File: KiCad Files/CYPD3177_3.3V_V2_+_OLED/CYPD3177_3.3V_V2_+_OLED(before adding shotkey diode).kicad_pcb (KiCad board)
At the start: 4 copper layers, 64 x 17 mm, 94 parts, among them IC1 TPS16630RGER, IC2 TPS22992SRXNR, J1 USB_C_USB2.0_16P, J2 Conn_01x02_Pin, J3 Conn_02x05_Odd_Even, J4 Conn_02x05_Odd_Even, J5 0.91 OLED, J6 QWIIC, J7 Conn_01x05, J8 I2C_Header, Q1 DMC2990UDJ-7, SW1 GT-TC0060-H050-L1, SW2 B3U-1000P, U1 TCA9406DC, U2 INA238, U3 XC6220B331PR-G, U4 TPS62933DRLR, U5 AON7534, U6 AP33772S, U7 AON7534, U8 TPS2117DRL, U9 ATtiny3217-M

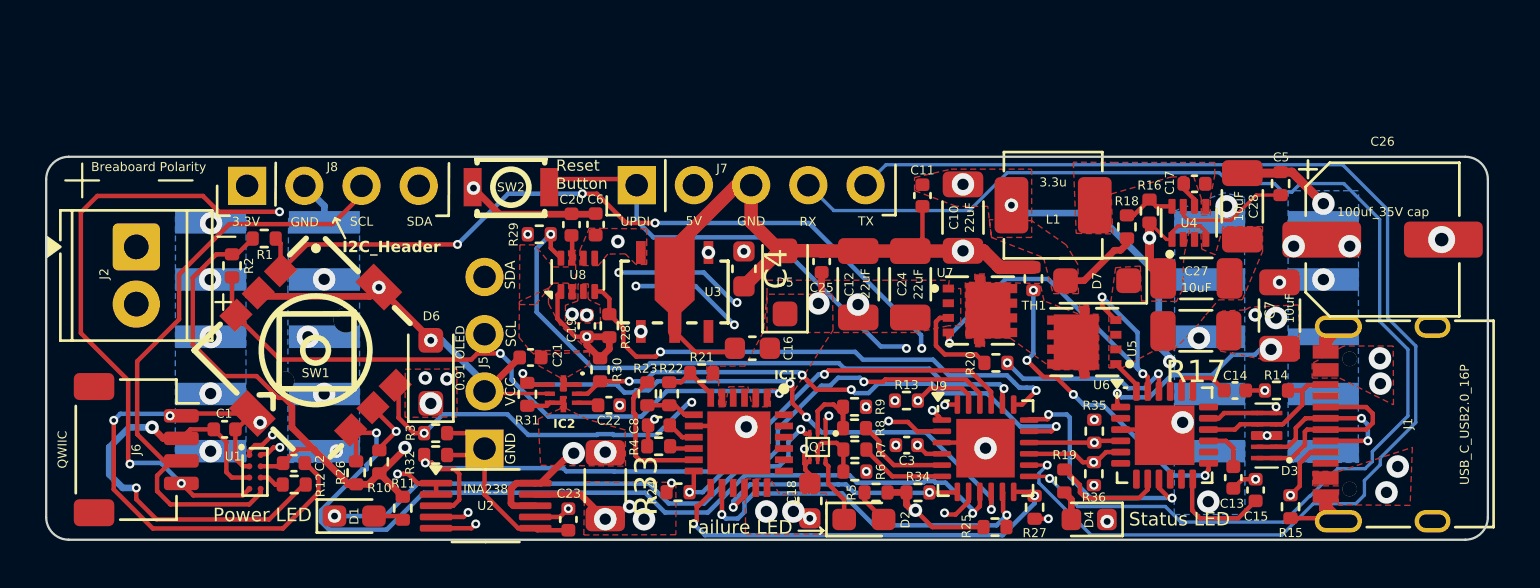
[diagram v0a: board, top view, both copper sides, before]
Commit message: changes
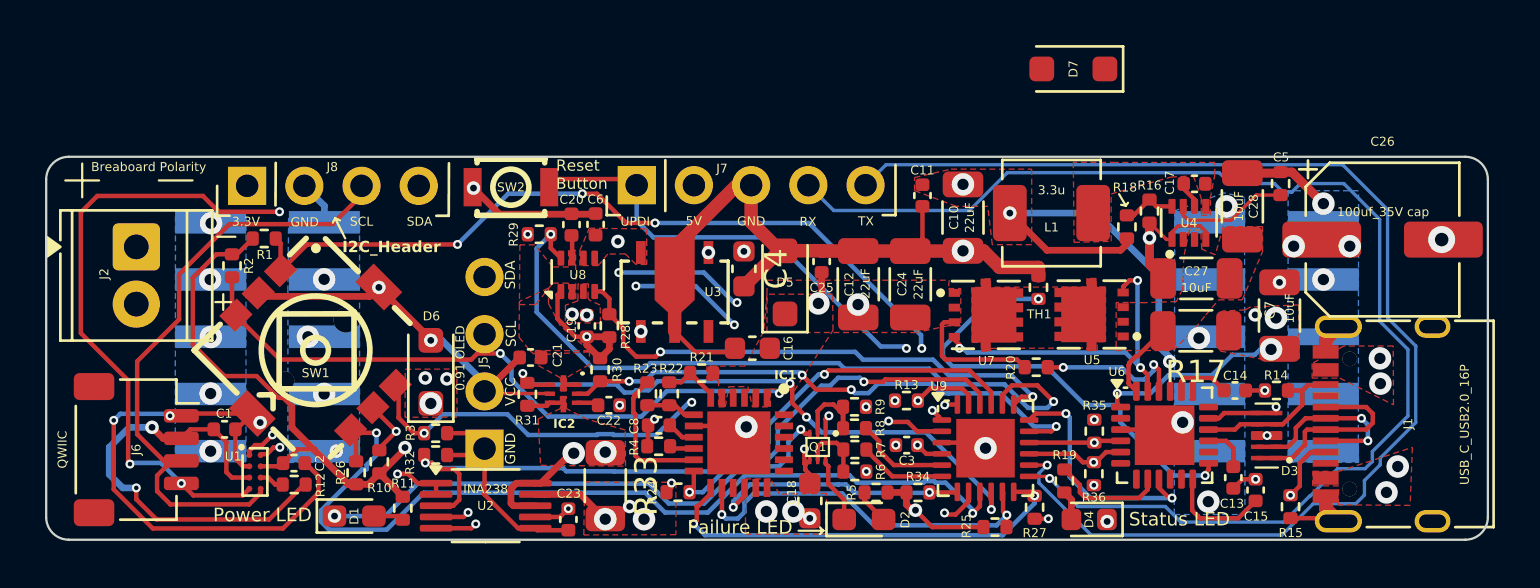
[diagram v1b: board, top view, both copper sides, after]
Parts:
- moved D7 9.46 mm to (144.6, 76.1)
- moved R20 1.80 mm to (142.9, 89.3)
- moved U5 1.27 mm to (145.4, 87.0)
- moved TH1 0.45 mm to (143.1, 85.8)
- moved L1 0.36 mm to (143.6, 82.5)
- moved U7 0.33 mm to (140.7, 87.0)
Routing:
- net /Power/NTC: track 13.9 -> 20.3 mm, vias 4 -> 2
- net /Logic/LOGIC_Report: track 28.0 -> 33.1 mm
- net Net-(U6-PWR_EN): track 18.6 -> 15.1 mm
- net +5V: track 92.7 -> 95.3 mm
- net /Power/Measured_VBUS: track 1.59 -> 3.65 mm
- net /Power/VBUS_Finale: track 13.9 -> 15.7 mm
- net Net-(U6-VOUT): track 8.24 -> 6.87 mm
- net GND: track 121.8 -> 122.3 mm
